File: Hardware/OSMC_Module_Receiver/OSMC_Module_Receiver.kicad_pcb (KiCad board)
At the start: 2 copper layers, 39 x 32 mm, 7 parts, among them J1 Conn_01x04_Socket, J2 Conn_01x04_Socket, J3 Conn_01x04_Socket, J4 Conn_01x04_Socket, J5 Conn_01x06_Pin

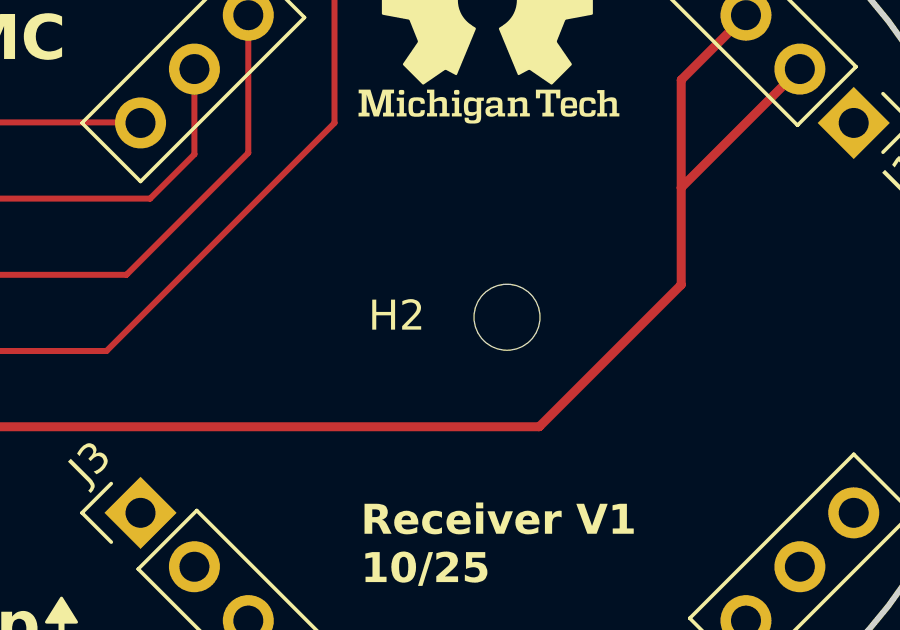
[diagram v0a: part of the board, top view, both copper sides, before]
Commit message: refile zones
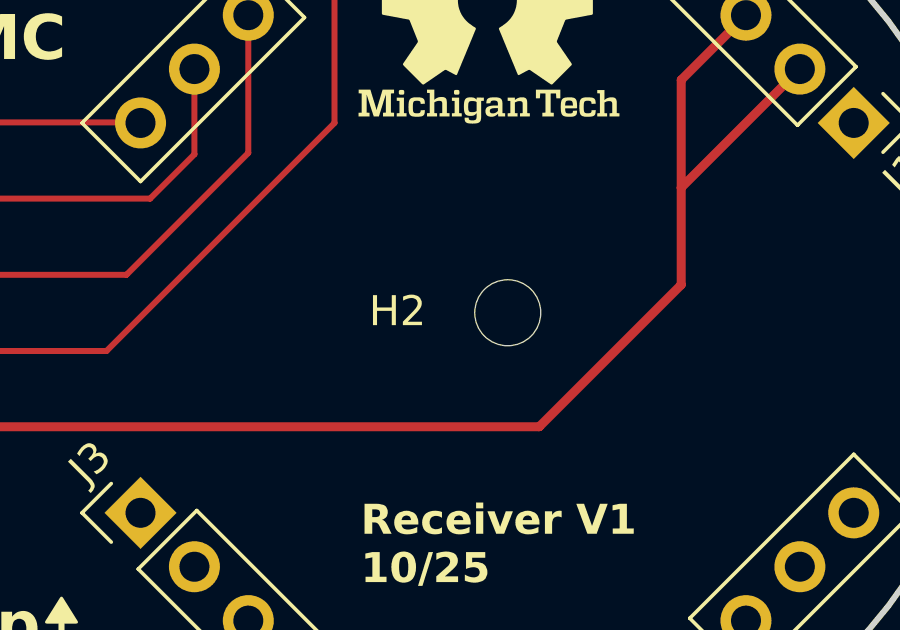
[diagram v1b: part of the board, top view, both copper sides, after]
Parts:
- moved H2 0.15 mm to (158.0, 61.0)
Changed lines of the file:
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@@
 	(footprint "MountingHole:MountingHole_2.2mm_M2"
 		(layer "F.Cu")
-		(at 157.975 61.125)
+		(at 158 60.975)
 		(descr "Mounting Hole 2.2mm, M2, no annular, generated by kicad-footprint-generator mountinghole.py")
 		(tags "mountinghole M2")
